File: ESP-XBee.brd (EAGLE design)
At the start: 10 parts, among them SW1 434111043826

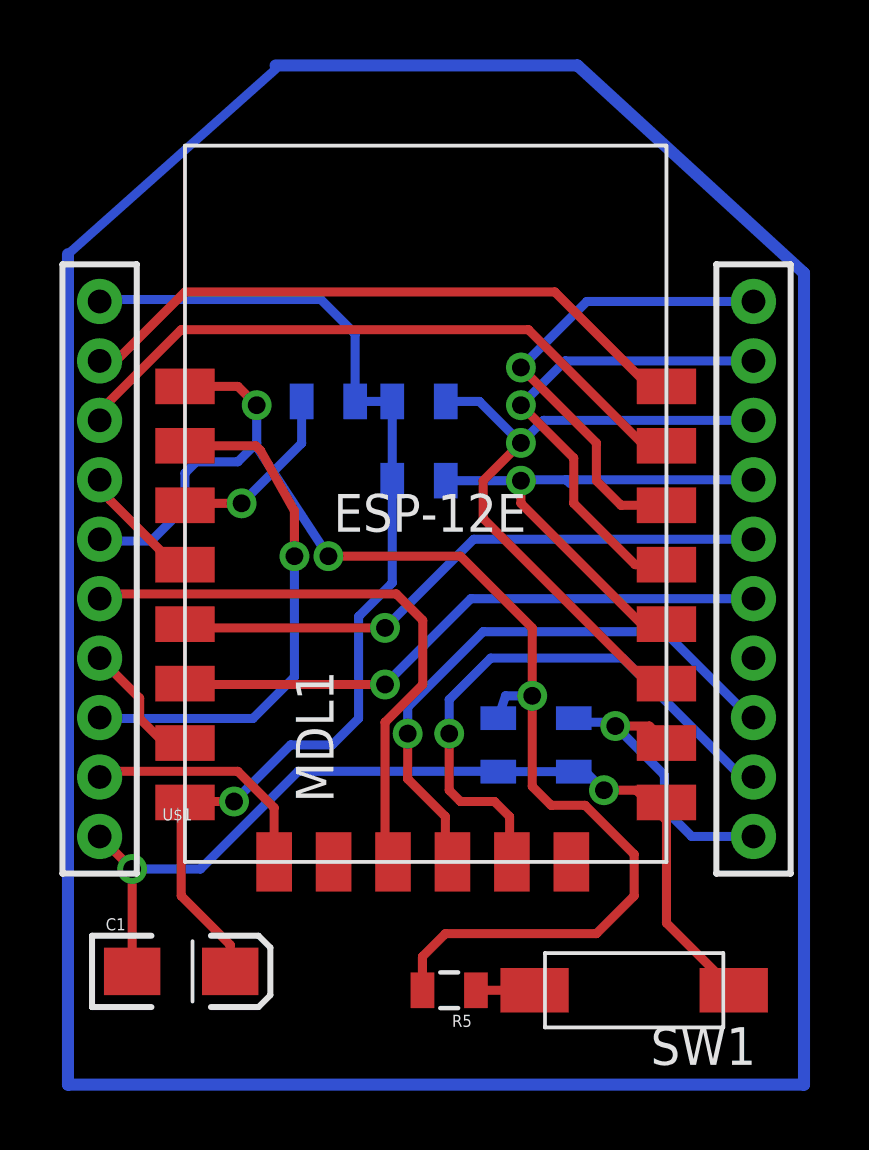
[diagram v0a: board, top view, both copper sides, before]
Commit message: seeedstudio GERBER generated
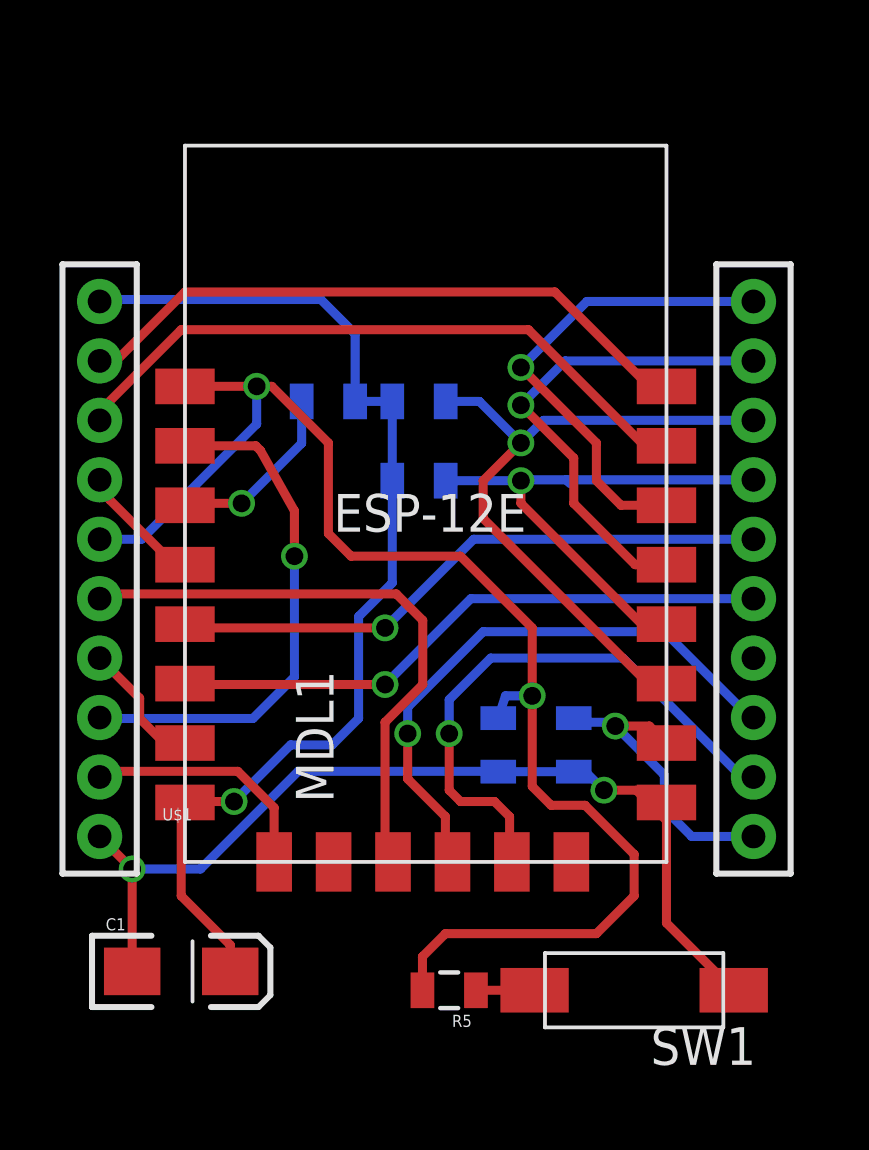
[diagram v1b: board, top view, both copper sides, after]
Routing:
- net N$2: track 109.9 -> 0.00 mm
- net RESET: track 45.6 -> 47.1 mm, vias 3 -> 2
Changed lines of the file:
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@@
 </class>
 </classes>
-<designrules name="default">
+<designrules name="SeeedStudio_2layer_DRU_no_angle_20140221">
 <description language="de">&lt;b&gt;EAGLE Design Rules&lt;/b&gt;
 &lt;p&gt;
@@
 necessary adjustments and save your customized
 design rules under a new name.</description>
+<description language="zh">&lt;b&gt;Seeed Studio EAGLE Design Rules&lt;/b&gt;
+</description>
 <param name="layerSetup" value="(1*16)"/>
-<param name="mtCopper" value="0.035mm 0.035mm 0.035mm 0.035mm 0.035mm 0.035mm 0.035mm 0.035mm 0.035mm 0.035mm 0.035mm 0.035mm 0.035mm 0.035mm 0.035mm 0.035mm"/>
-<param name="mtIsolate" value="1.5mm 0.15mm 0.2mm 0.15mm 0.2mm 0.15mm 0.2mm 0.15mm 0.2mm 0.15mm 0.2mm 0.15mm 0.2mm 0.15mm 0.2mm"/>
-<param name="mdWireWire" value="8mil"/>
-<param name="mdWirePad" value="8mil"/>
-<param name="mdWireVia" value="8mil"/>
-<param name="mdPadPad" value="8mil"/>
-<param name="mdPadVia" value="8mil"/>
-<param name="mdViaVia" value="8mil"/>
-<param name="mdSmdPad" value="8mil"/>
-<param name="mdSmdVia" value="8mil"/>
-<param name="mdSmdSmd" value="8mil"/>
+<param name="mtCopper" value="0.035mm 0.0175mm 0.035mm 0.035mm 0.035mm 0.035mm 0.035mm 0.035mm 0.035mm 0.035mm 0.035mm 0.035mm 0.035mm 0.035mm 0.0175mm 0.035mm"/>
+<param name="mtIsolate" value="1.5mm 1.1mm 0.2mm 0.15mm 0.2mm 0.15mm 0.2mm 0.15mm 0.2mm 0.15mm 0.2mm 0.15mm 0.2mm 0.15mm 0.2mm"/>
+<param name="mdWireWire" value="6mil"/>
+<param name="mdWirePad" value="6mil"/>
+<param name="mdWireVia" value="6mil"/>
+<param name="mdPadPad" value="6mil"/>
+<param name="mdPadVia" value="6mil"/>
+<param name="mdViaVia" value="6mil"/>
+<param name="mdSmdPad" value="0mil"/>
+<param name="mdSmdVia" value="0mil"/>
+<param name="mdSmdSmd" value="0mil"/>
 <param name="mdViaViaSameLayer" value="8mil"/>
 <param name="mnLayersViaInSmd" value="2"/>
-<param name="mdCopperDimension" value="40mil"/>
-<param name="mdDrill" value="8mil"/>
+<param name="mdCopperDimension" value="10mil"/>
+<param name="mdDrill" value="10mil"/>
 <param name="mdSmdStop" value="0mil"/>
-<param name="msWidth" value="10mil"/>
-<param name="msDrill" value="24mil"/>
-<param name="msMicroVia" value="9.99mm"/>
+<param name="msWidth" value="6mil"/>
+<param name="msDrill" value="12mil"/>
+<param name="msMicroVia" value="12mil"/>
 <param name="msBlindViaRatio" value="0.5"/>
 <param name="rvPadTop" value="0.25"/>
@@
 <param name="rlMinPadBottom" value="10mil"/>
 <param name="rlMaxPadBottom" value="20mil"/>
-<param name="rlMinViaOuter" value="8mil"/>
+<param name="rlMinViaOuter" value="6mil"/>
 <param name="rlMaxViaOuter" value="20mil"/>
-<param name="rlMinViaInner" value="8mil"/>
+<param name="rlMinViaInner" value="6mil"/>
 <param name="rlMaxViaInner" value="20mil"/>
 <param name="rlMinMicroViaOuter" value="4mil"/>
@@
 <param name="psTop" value="-1"/>
 <param name="psBottom" value="-1"/>
-<param name="psFirst" value="-1"/>
+<param name="psFirst" value="0"/>
 <param name="psElongationLong" value="100"/>
 <param name="psElongationOffset" value="100"/>
 <param name="mvStopFrame" value="1"/>
 <param name="mvCreamFrame" value="0"/>
-<param name="mlMinStopFrame" value="4mil"/>
-<param name="mlMaxStopFrame" value="4mil"/>
+<param name="mlMinStopFrame" value="2mil"/>
+<param name="mlMaxStopFrame" value="2mil"/>
 <param name="mlMinCreamFrame" value="0mil"/>
 <param name="mlMaxCreamFrame" value="0mil"/>
-<param name="mlViaStopLimit" value="0mil"/>
+<param name="mlViaStopLimit" value="100mil"/>
 <param name="srRoundness" value="0"/>
 <param name="srMinRoundness" value="0mil"/>
@@
 <param name="checkAngle" value="0"/>
 <param name="checkFont" value="1"/>
-<param name="checkRestrict" value="1"/>
+<param name="checkRestrict" value="0"/>
 <param name="useDiameter" value="13"/>
 <param name="maxErrors" value="50"/>
@@
 <contactref element="C2" pad="1"/>
 <contactref element="R5" pad="2"/>
-<wire x1="34.417" y1="42.543" x2="36.197" y2="42.543" width="0.3048" layer="1"/>
-<wire x1="36.197" y1="42.543" x2="36.83" y2="41.91" width="0.3048" layer="1"/>
-<via x="36.83" y="41.91" extent="1-16" drill="0.6" shape="octagon"/>
-<wire x1="36.83" y1="41.91" x2="36.83" y2="40.64" width="0.3048" layer="16"/>
-<wire x1="36.83" y1="40.64" x2="36.195" y2="40.005" width="0.3048" layer="16"/>
-<wire x1="36.195" y1="40.005" x2="34.798" y2="40.005" width="0.3048" layer="16"/>
-<wire x1="34.798" y1="40.005" x2="34.417" y2="39.624" width="0.3048" layer="16"/>
-<wire x1="34.417" y1="39.624" x2="34.417" y2="38.481" width="0.3048" layer="16"/>
-<wire x1="34.417" y1="38.481" x2="33.274" y2="37.338" width="0.3048" layer="16"/>
-<wire x1="33.274" y1="37.338" x2="31.607" y2="37.338" width="0.3048" layer="16"/>
-<wire x1="31.607" y1="37.338" x2="31.545" y2="37.4" width="0.3048" layer="16"/>
 <wire x1="42.407" y1="22.225" x2="42.407" y2="23.357" width="0.3048" layer="1"/>
 <wire x1="42.407" y1="23.357" x2="43.18" y2="24.13" width="0.3048" layer="1"/>
@@
 <wire x1="46.101" y1="32.131" x2="45.201" y2="32.131" width="0.3048" layer="16"/>
 <wire x1="45.201" y1="32.131" x2="44.958" y2="31.38" width="0.3048" layer="16"/>
-<wire x1="36.83" y1="40.64" x2="36.83" y2="40.513" width="0.3048" layer="16"/>
-<wire x1="36.83" y1="40.513" x2="39.243" y2="36.83" width="0.3048" layer="16"/>
-<via x="39.243" y="36.83" extent="1-16" drill="0.6" shape="octagon"/>
-<wire x1="39.243" y1="36.83" x2="43.688" y2="36.83" width="0.3048" layer="1"/>
 <wire x1="43.688" y1="36.83" x2="46.101" y2="34.417" width="0.3048" layer="1"/>
 <wire x1="46.101" y1="34.417" x2="46.101" y2="32.131" width="0.3048" layer="1"/>
+<wire x1="43.688" y1="36.83" x2="40.005" y2="36.83" width="0.3048" layer="1"/>
+<wire x1="40.005" y1="36.83" x2="39.243" y2="37.592" width="0.3048" layer="1"/>
+<wire x1="39.243" y1="37.592" x2="39.243" y2="40.64" width="0.3048" layer="1"/>
+<wire x1="31.545" y1="37.4" x2="32.955" y2="37.4" width="0.3048" layer="16"/>
+<wire x1="32.955" y1="37.4" x2="36.83" y2="41.275" width="0.3048" layer="16"/>
+<wire x1="34.542" y1="42.418" x2="34.417" y2="42.543" width="0.3048" layer="1"/>
+<wire x1="36.83" y1="41.275" x2="36.83" y2="42.545" width="0.3048" layer="16"/>
+<via x="36.83" y="42.545" extent="1-16" drill="0.6" shape="octagon"/>
+<wire x1="36.83" y1="42.545" x2="34.419" y2="42.545" width="0.3048" layer="1"/>
+<wire x1="34.419" y1="42.545" x2="34.417" y2="42.543" width="0.3048" layer="1"/>
+<wire x1="39.243" y1="40.64" x2="37.338" y2="42.545" width="0.3048" layer="1"/>
+<wire x1="37.338" y1="42.545" x2="36.83" y2="42.545" width="0.3048" layer="1"/>
 </signal>
 <signal name="ADC">
@@
 <wire x1="46.18" y1="22.225" x2="44.207" y2="22.225" width="0.3048" layer="1"/>
 </signal>
-<signal name="N$2">
-<wire x1="30.48" y1="19.05" x2="55.245" y2="19.05" width="0.4064" layer="16"/>
-<wire x1="55.245" y1="19.05" x2="55.245" y2="46.355" width="0.4064" layer="16"/>
-<wire x1="55.245" y1="46.355" x2="47.625" y2="53.34" width="0.4064" layer="16"/>
-<wire x1="47.625" y1="53.34" x2="37.465" y2="53.34" width="0.4064" layer="16"/>
-<wire x1="30.48" y1="46.99" x2="30.48" y2="19.05" width="0.4064" layer="16"/>
-<wire x1="30.48" y1="46.99" x2="37.465" y2="53.213" width="0.3048" layer="16"/>
-</signal>
 </signals>
